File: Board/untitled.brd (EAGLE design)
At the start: 142.9 x 168.6 mm, 109 parts, among them IC1 74HC595N, IC2 74HC595N, IC3 74HC595N, IC4 74HC595N, IC5 74HC595N, IC6 74HC595N, IC7 74HC595N, IC8 74HC595N, IC9 74HC595N, J1 DCJ0202, Q1 BC447, Q2 BC447, Q3 BC447, T1 TIP122, T2 TIP122, T3 TIP122, T4 TIP122, T5 TIP122, T6 TIP122, T7 TIP122, T8 TIP122

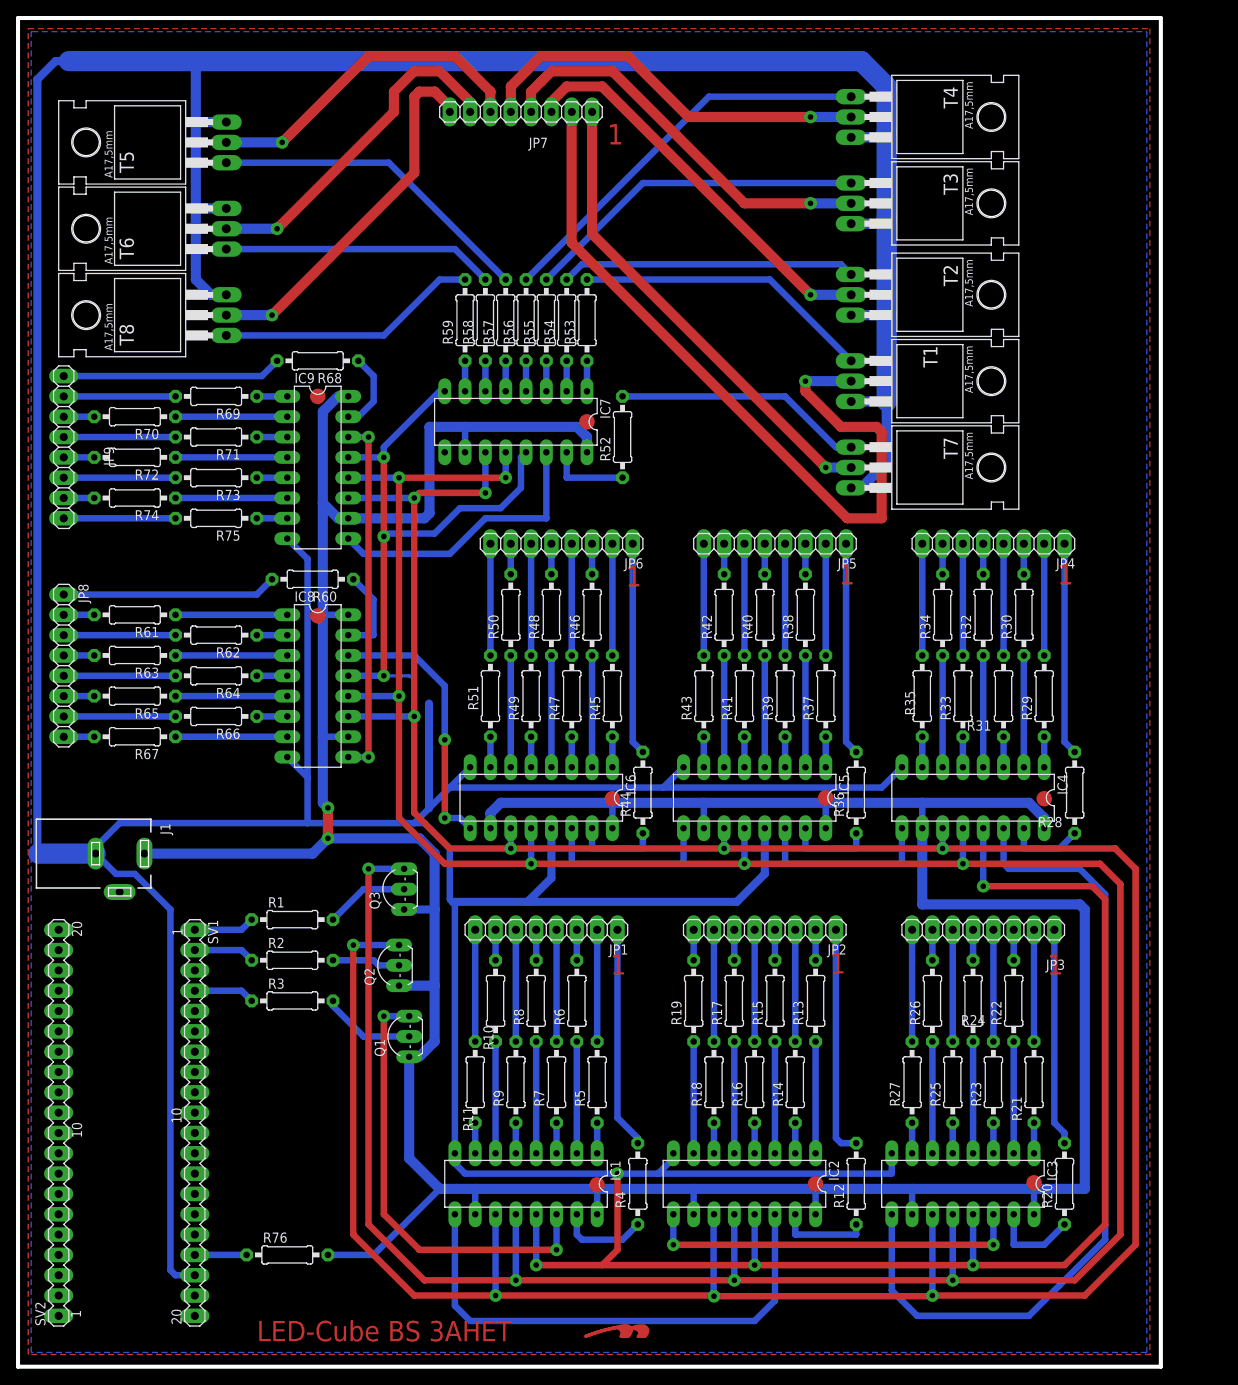
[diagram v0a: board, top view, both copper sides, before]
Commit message: new board
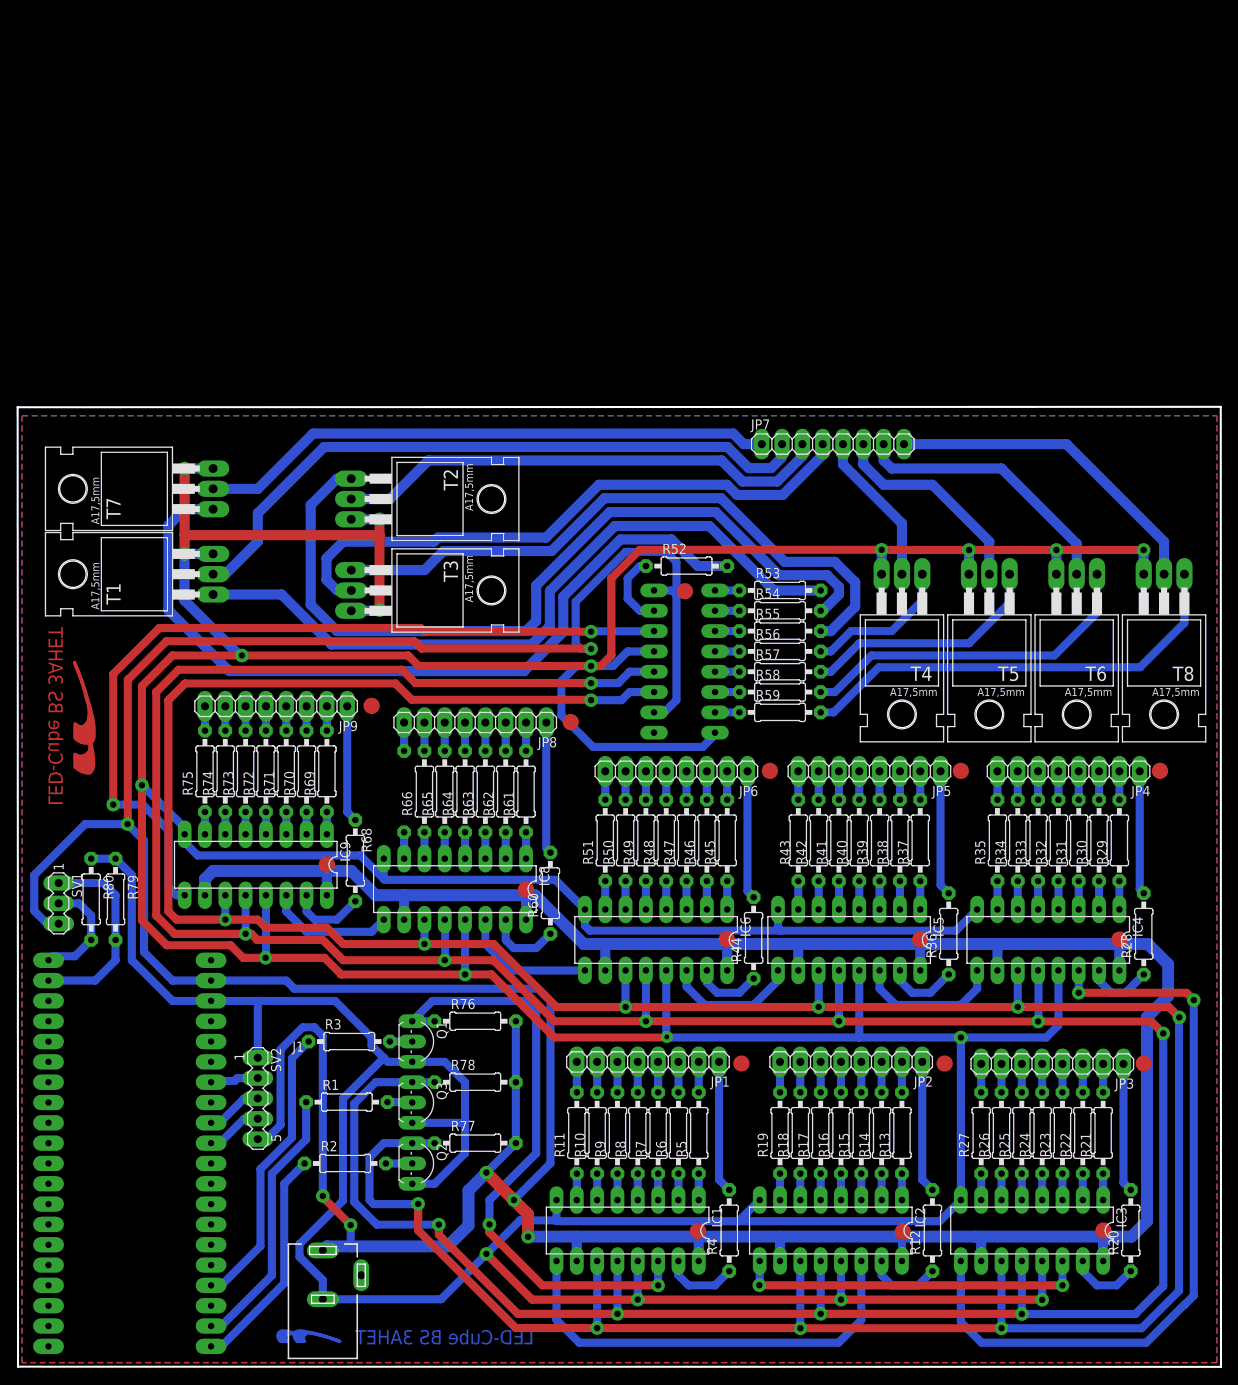
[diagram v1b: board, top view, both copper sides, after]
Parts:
- added R77, R78, R79, R80: (no value), rcl:0207/10
- added U$2: (no value), PI_PICO:PI_PICO
- added U$3: (no value), HTL-Logo:LOGOTOP_15
- SV1: device con-lstb:MA20-1 -> con-lstb:MA03-1
- SV2: device con-lstb:MA20-1 -> con-lstb:MA05-1
- U$1: device HTL-Logo:LOGOTOP_8 -> HTL-Logo:LOGOBOT_8
- moved T8 129.5 mm to (143.3, 92.7), turned to 180 degrees
- moved T6 123.1 mm to (132.3, 92.7), turned to 180 degrees
- moved T5 118.3 mm to (121.4, 92.7), turned to 180 degrees
- moved T1 95.6 mm to (18.0, 99.1), turned to 90 degrees
- moved T7 92.5 mm to (18.0, 109.7), turned to 90 degrees
- moved T3 79.0 mm to (48.0, 97.0)
- moved T2 67.5 mm to (48.0, 108.5)
- moved T4 63.5 mm to (110.5, 92.7), turned to 180 degrees
- moved R59 62.9 mm to (95.2, 81.8), turned to 0 degrees
- moved R68 62.7 mm to (42.2, 63.2), turned to 90 degrees
- moved R58 59.3 mm to (95.2, 84.3), turned to 0 degrees
- moved J1 58.5 mm to (38.1, 11.4), turned to 0 degrees
- moved JP7 57.0 mm to (101.9, 115.3), turned to 0 degrees
- moved R57 55.7 mm to (95.2, 86.9), turned to 0 degrees
- moved R61 53.7 mm to (63.5, 71.9), turned to 90 degrees
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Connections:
- new net DATA: IC1.14, Q1.C, R76.1
- new net N$153: SV2.2, U$2.GP28
- new net SHIFT: IC1.11, IC2.11, IC3.11, IC4.11, IC5.11, IC6.11, IC7.11, IC8.11, IC9.11, Q2.C, R77.1
- new net STORE: IC1.12, IC2.12, IC3.12, IC4.12, IC5.12, IC6.12, IC7.12, IC8.12, IC9.12, Q3.C, R78.1
- net GND: now also Q1.E, Q2.E, Q3.E, R79.1, R80.1, SV2.1, U$2.GND8; no longer SV1.18
- net N$1: now also U$2.GP17; no longer SV1.1
- net N$118: now also SV2.3, U$2.GP27; no longer R76.1, SV1.17
- net N$3: now also SV2.4, U$2.GP26; no longer R3.1, SV1.4
- net N$41: now also R80.2, SV1.2, U$2.GP0; no longer IC1.14, Q1.E
- net N$43: now also R79.2, SV1.1, U$2.GP1; no longer IC1.12, IC2.12, IC3.12, IC4.12, IC5.12, IC6.12, IC7.12, IC8.12, IC9.12, Q3.E
- net N$6: now also R3.1, U$2.GP18; no longer R2.1, SV1.2
- net N$7: now also R2.1, U$2.GP16; no longer IC1.11, IC2.11, IC3.11, IC4.11, IC5.11, IC6.11, IC7.11, IC8.11, IC9.11, Q2.E
- net VCC: now also R77.2, R78.2, SV1.3, SV2.5, U$2.VSYS; no longer Q1.C, Q2.C, Q3.C
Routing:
- net STORE: track 0.00 -> 437.6 mm, vias 0 -> 11
- net SHIFT: track 0.00 -> 426.3 mm, vias 0 -> 11
- net N$43: track 395.4 -> 25.3 mm, vias 10 -> 0
- net N$7: track 394.0 -> 28.4 mm, vias 10 -> 0
- net VCC: track 477.4 -> 636.9 mm, vias 2 -> 7
- net DATA: track 0.00 -> 76.8 mm, vias 0 -> 2
- net N$120: track 31.2 -> 100.8 mm
- net N$173: track 35.7 -> 104.3 mm, vias 0 -> 2
- net N$122: track 36.9 -> 103.0 mm
- net N$121: track 37.2 -> 90.6 mm
- net GND: track 957.1 -> 906.2 mm, vias 8 -> 19
- net N$41: track 55.8 -> 14.1 mm, vias 2 -> 0
- net N$123: track 43.1 -> 79.7 mm
- net N$124: track 50.1 -> 18.6 mm
- net N$132: track 50.5 -> 19.3 mm, vias 1 -> 0
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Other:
- board size 142.9 x 168.6 mm -> 150.4 x 120 mm
- board text removed: "1"
